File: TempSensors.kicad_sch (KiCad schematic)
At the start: 38 parts, among them IC1 TLV9002QDRQ1, IC2 TLV9002QDRQ1, U3 TLV9002QDRQ1, U4 TLV9002QDRQ1

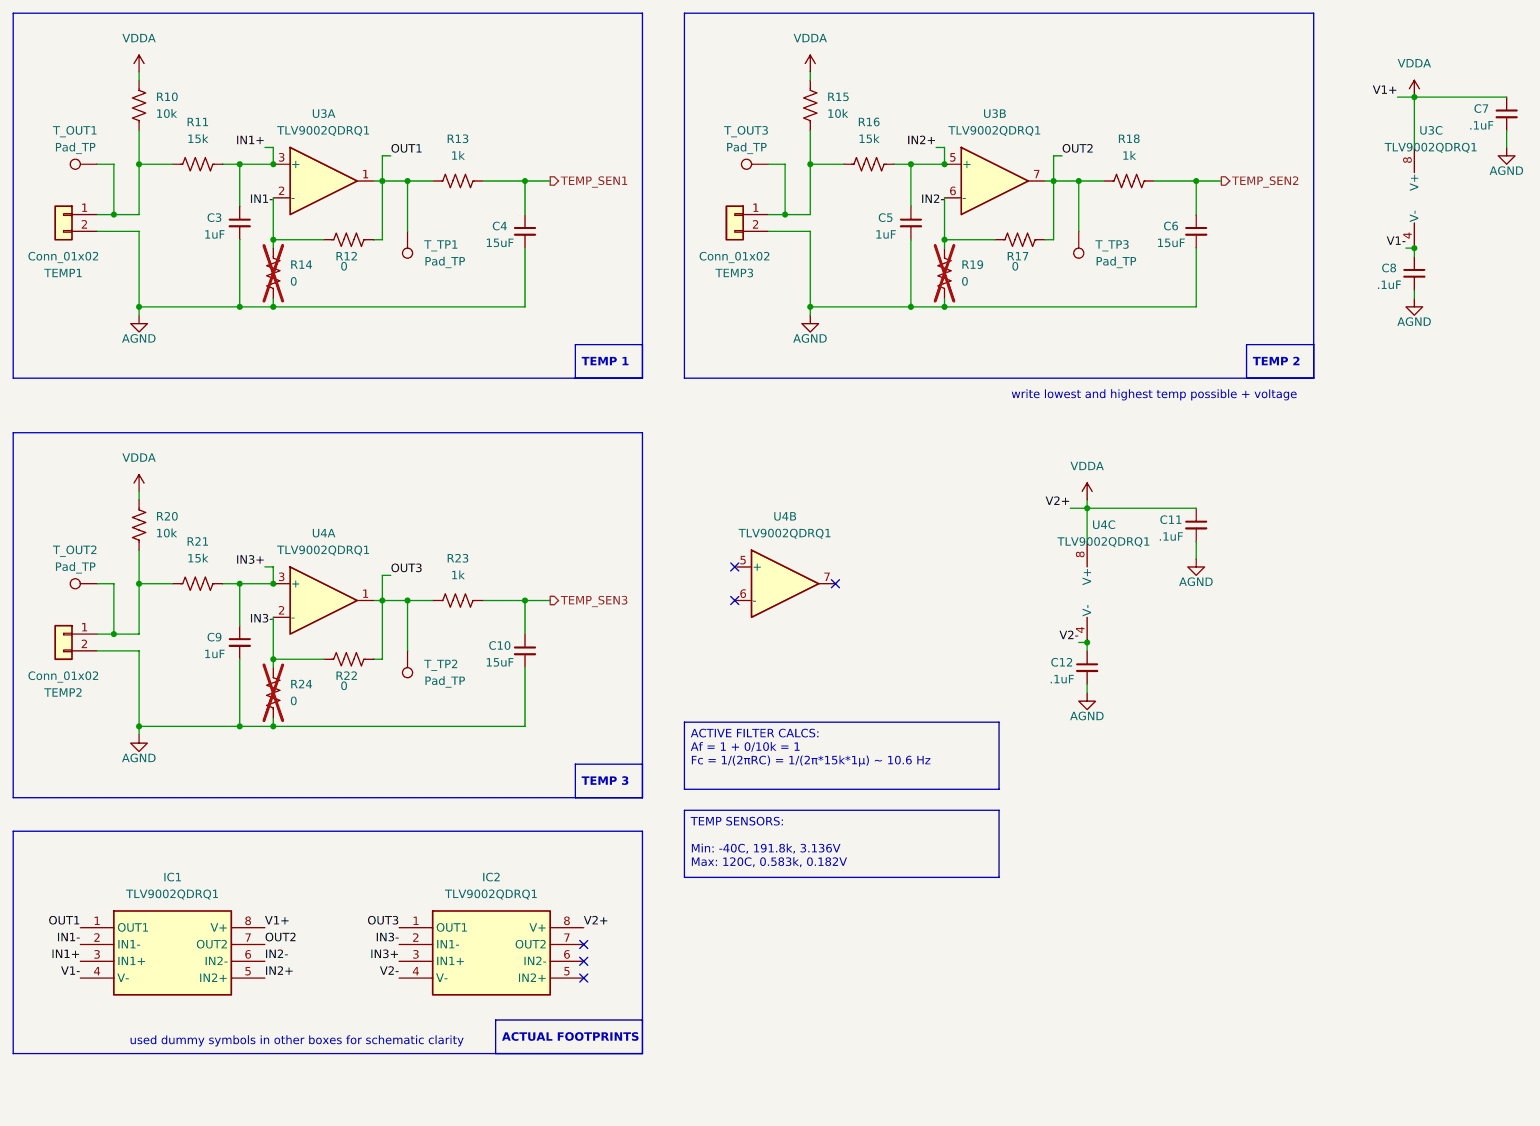
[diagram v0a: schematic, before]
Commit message: fixed submodule, schematic basically done
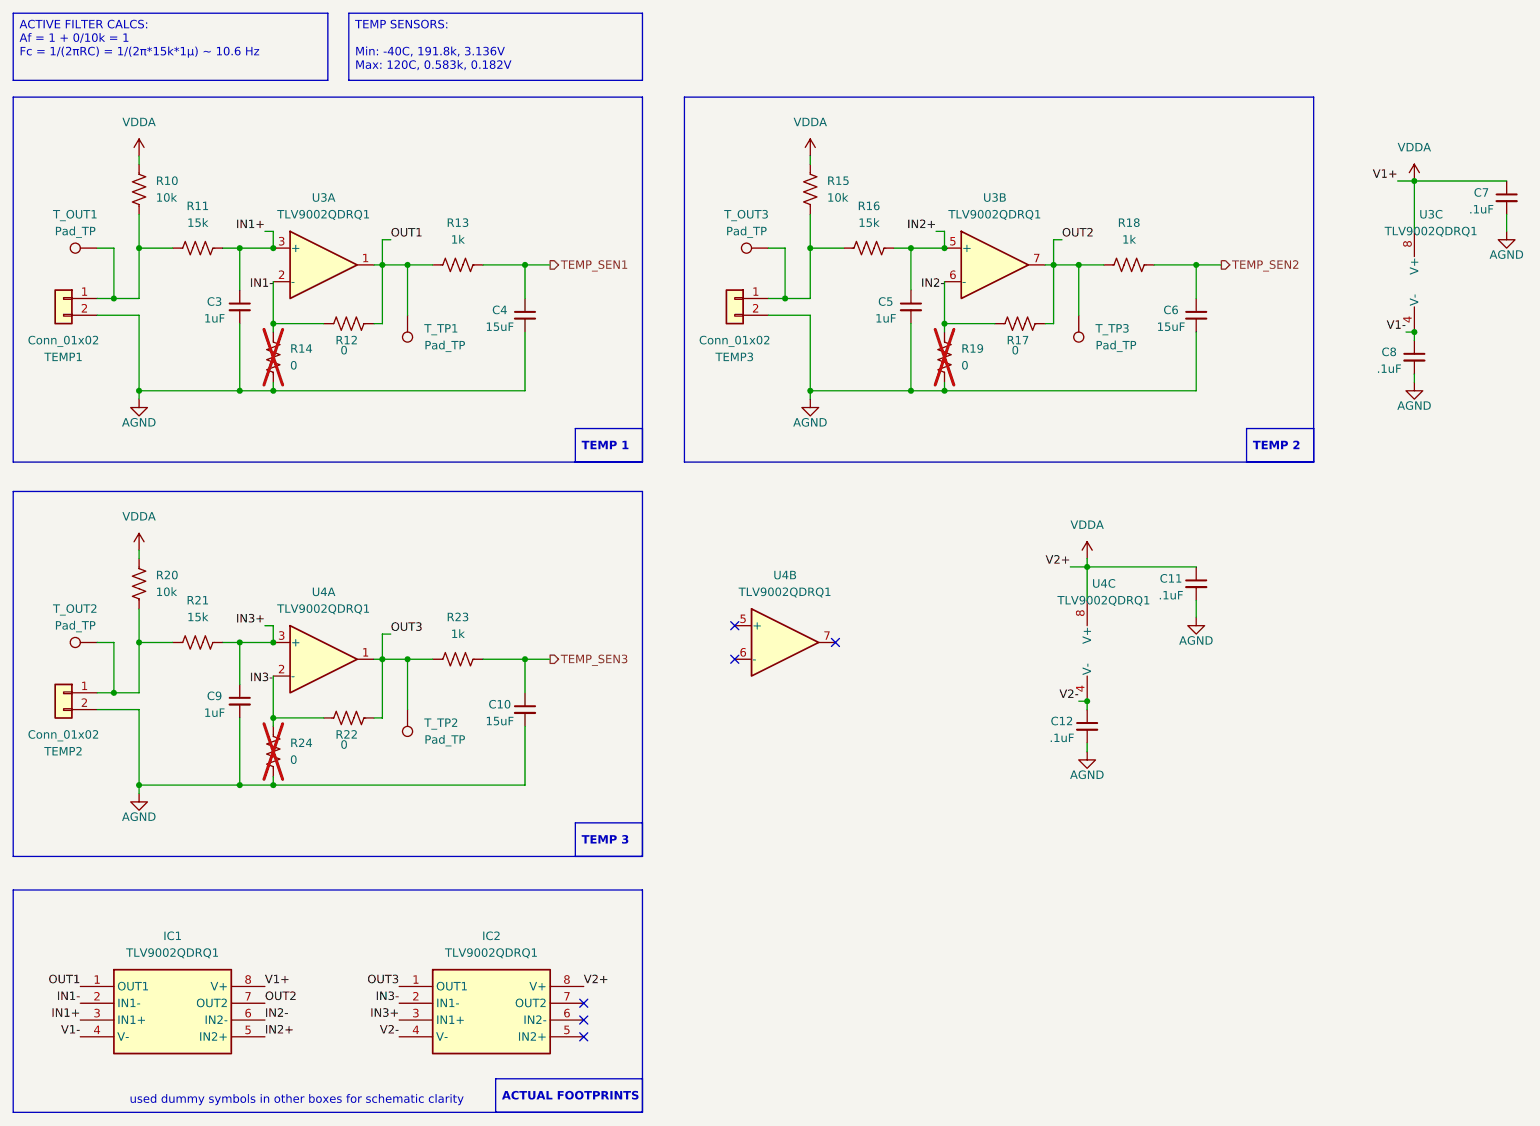
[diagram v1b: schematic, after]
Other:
- note removed: "write lowest and highest temp possible + voltage"
- moved on the sheet: C10, C11, C12, C3, C4, C5, C6, C7, C8, C9, IC1, IC2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
